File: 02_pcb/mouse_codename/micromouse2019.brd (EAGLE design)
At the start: 45 x 50 mm, 75 parts

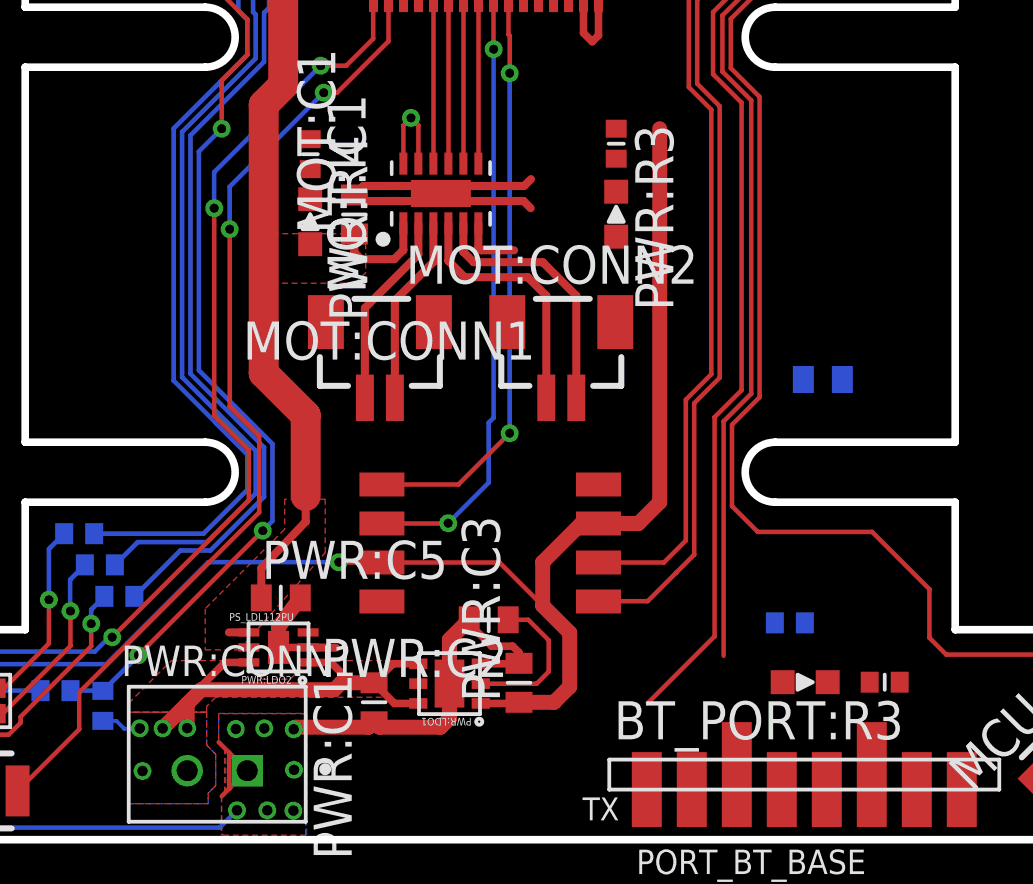
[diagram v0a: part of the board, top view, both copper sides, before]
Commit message: lib updated
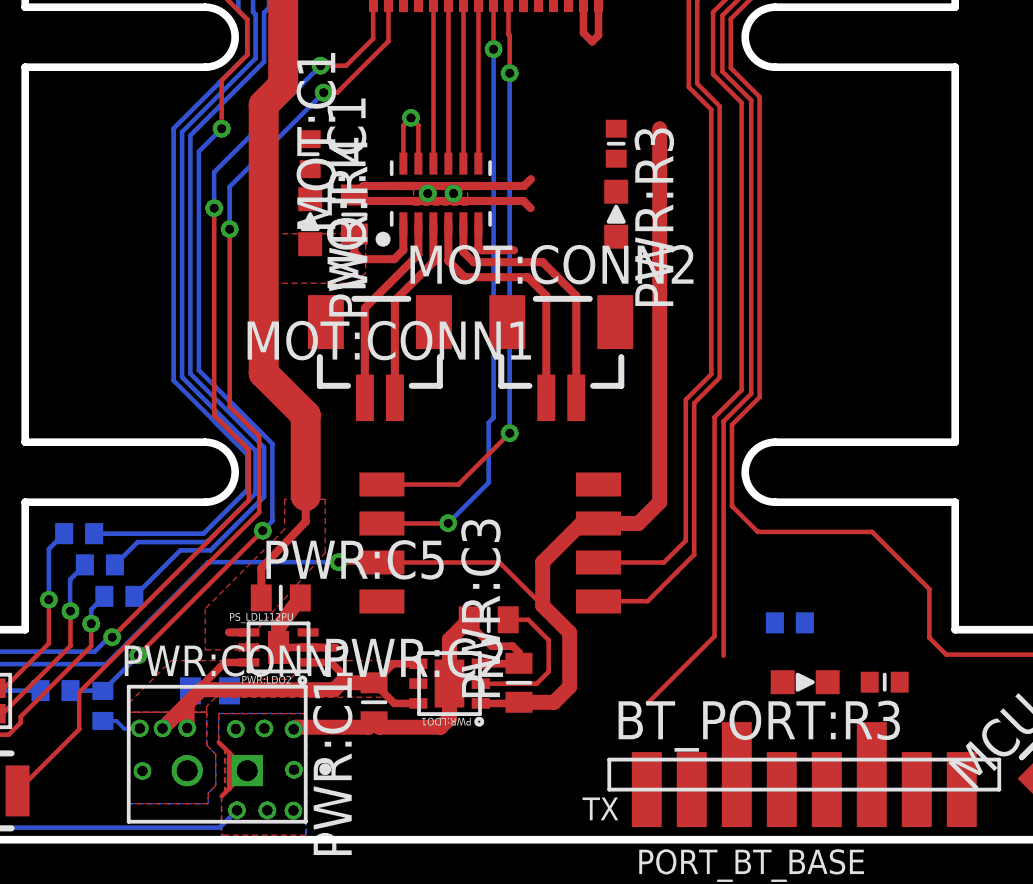
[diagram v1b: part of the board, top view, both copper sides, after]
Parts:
- moved PWR:C4 22.9 mm to (13.2, 4.96), turned to 180 degrees
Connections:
- net GND: no longer MOT:IC1.13
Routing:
- net GND: track 58.2 -> 67.9 mm, vias 8 -> 10
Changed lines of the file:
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@@
 <drawing>
 <settings>
-<setting alwaysvectorfont="yes"/>
+<setting alwaysvectorfont="no"/>
 <setting verticaltext="up"/>
 </settings>
@@
 <attribute name="VALUE" x="25.365" y="4.595" size="1.27" layer="27" rot="R90"/>
 </element>
-<element name="PWR:C4" library="0-micromouse2019" package="C0402" package3d_urn="urn:adsk.eagle:package:23626/2" value="1u" x="33.59" y="15.34" smashed="yes" rot="MR0">
-<attribute name="NAME" x="34.225" y="15.975" size="1.27" layer="26" rot="MR0"/>
-<attribute name="SPICEPREFIX" value="C" x="33.59" y="15.34" size="1.778" layer="28" rot="MR0" display="off"/>
-<attribute name="VALUE" x="34.225" y="13.435" size="1.27" layer="28" rot="MR0"/>
+<element name="PWR:C4" library="0-micromouse2019" package="C0402" package3d_urn="urn:adsk.eagle:package:23626/2" value="1u" x="13.16" y="4.96" smashed="yes" rot="MR180">
+<attribute name="NAME" x="12.525" y="4.325" size="1.27" layer="26" rot="MR180"/>
+<attribute name="SPICEPREFIX" value="C" x="13.16" y="4.96" size="1.778" layer="28" rot="MR180" display="off"/>
+<attribute name="VALUE" x="12.525" y="6.865" size="1.27" layer="28" rot="MR180"/>
 </element>
 <element name="PWR:C5" library="0-micromouse2019" package="C0402" package3d_urn="urn:adsk.eagle:package:23626/2" value="10u" x="15.52" y="8.06" smashed="yes">
@@
 <contactref element="MCU:J1" pad="3"/>
 <contactref element="MOT:C1" pad="2"/>
-<contactref element="MOT:IC1" pad="13"/>
 <contactref element="MOT:IC1" pad="14"/>
 <contactref element="MOT:IC1" pad="16"/>
@@
 <wire x1="15.45" y1="7.1" x2="16.17" y2="8.06" width="0.5" layer="1"/>
 <wire x1="16.4315" y1="6.409" x2="17.35" y2="6.4" width="0.27" layer="1"/>
-<polygon width="0.1524" layer="16" pour="cutout" rank="3">
+<polygon width="0.1524" layer="16" pour="cutout" isolate="0.3048" rank="3">
 <vertex x="0" y="0"/>
 <vertex x="45" y="0"/>
@@
 <contactref element="MCU:R8" pad="2"/>
 <contactref element="MCU:R9" pad="2"/>
+<via x="20.42" y="21.54" extent="1-16" drill="0.3" diameter="0.6"/>
+<via x="21.28" y="21.54" extent="1-16" drill="0.3" diameter="0.6"/>
+<polygon width="0.1" layer="1" spacing="0.5" isolate="0.254">
+<vertex x="19.95" y="21.9"/>
+<vertex x="21.75" y="21.9"/>
+<vertex x="21.75" y="21.15"/>
+<vertex x="19.95" y="21.15"/>
+</polygon>
+<wire x1="19.4874" y1="21.29" x2="22.2246" y2="21.29" width="0.27" layer="1"/>
+<wire x1="19.4874" y1="21.79" x2="22.2246" y2="21.79" width="0.27" layer="1"/>
+<wire x1="22.2246" y1="21.29" x2="21.53" y2="21.29" width="0.27" layer="1"/>
+<wire x1="21.53" y1="21.29" x2="21.285" y2="21.535" width="0.27" layer="1"/>
+<wire x1="21.285" y1="21.535" x2="21.28" y2="21.54" width="0.27" layer="1"/>
+<wire x1="22.2246" y1="21.79" x2="21.54" y2="21.79" width="0.27" layer="1"/>
+<wire x1="21.54" y1="21.79" x2="21.285" y2="21.535" width="0.27" layer="1"/>
+<wire x1="20.42" y1="21.54" x2="20.17" y2="21.29" width="0.27" layer="1"/>
+<wire x1="20.17" y1="21.29" x2="19.4874" y2="21.29" width="0.27" layer="1"/>
+<wire x1="20.42" y1="21.54" x2="20.17" y2="21.79" width="0.27" layer="1"/>
+<wire x1="20.17" y1="21.79" x2="19.4874" y2="21.79" width="0.27" layer="1"/>
 <wire x1="38" y1="36.7" x2="38" y2="38.3" width="0" layer="19" extent="16-16"/>
 <wire x1="38" y1="40" x2="38" y2="38.3" width="0" layer="19" extent="16-16"/>
@@
 <wire x1="9.8" y1="47.7" x2="9.75" y2="46.2" width="0" layer="19" extent="16-16"/>
 <wire x1="16.5" y1="23.35" x2="18.54" y2="28.74" width="0" layer="19" extent="1-16"/>
-<wire x1="18.273" y1="21.79" x2="16.5" y2="23.35" width="0" layer="19" extent="1-1"/>
-<wire x1="20.856" y1="21.54" x2="19.4874" y2="21.79" width="0" layer="19" extent="1-1"/>
-<wire x1="22.2246" y1="21.79" x2="20.856" y2="21.54" width="0" layer="19" extent="1-1"/>
-<wire x1="23.61" y1="21.29" x2="23.63" y2="21.79" width="0" layer="19" extent="1-1"/>
+<wire x1="17.973" y1="21.49" x2="16.5" y2="23.35" width="0" layer="19" extent="1-1"/>
 <wire x1="22.106" y1="20.5444" x2="22.2246" y2="21.29" width="0" layer="19" extent="1-1"/>
 <wire x1="26.7" y1="23.7" x2="23.86" y2="22.02" width="0" layer="19" extent="1-1"/>
 <wire x1="26.11" y1="11.84" x2="23.297" y2="19.647" width="0" layer="19" extent="1-1"/>
 <wire x1="23.25" y1="6.45" x2="26.11" y2="11.84" width="0" layer="19" extent="1-1"/>
-<wire x1="18.89" y1="7.94" x2="21.144" y2="6.674" width="0" layer="19" extent="1-1"/>
-<wire x1="17.35" y1="6.4" x2="18.89" y2="7.94" width="0" layer="19" extent="1-1"/>
-<wire x1="32.94" y1="15.34" x2="26.11" y2="11.84" width="0" layer="19" extent="1-16"/>
+<wire x1="13.81" y1="4.96" x2="14.02" y2="3.69" width="0" layer="19" extent="16-16"/>
+<wire x1="15.444" y1="6.409" x2="13.81" y2="4.96" width="0" layer="19" extent="1-16"/>
+<wire x1="18.89" y1="7.94" x2="17.35" y2="6.4" width="0" layer="19" extent="1-1"/>
 <wire x1="15.75" y1="56.8" x2="20.385" y2="48.379" width="0" layer="19" extent="1-16"/>
 <wire x1="14.7" y1="56.8" x2="15.75" y2="56.8" width="0" layer="19" extent="16-16"/>
 <wire x1="13.6" y1="56.8" x2="14.7" y2="56.8" width="0" layer="19" extent="16-16"/>
-<wire x1="36.15" y1="5.25" x2="32.94" y2="15.34" width="0" layer="19" extent="1-16"/>
+<wire x1="36.15" y1="5.25" x2="26.11" y2="11.84" width="0" layer="19" extent="1-1"/>
 <wire x1="36.72" y1="1.67" x2="36.15" y2="5.25" width="0" layer="19" extent="1-1"/>
 </signal>
@@
 <contactref element="PWR:LDO1" pad="4"/>
 <contactref element="PWR:LDO1" pad="6"/>
-<wire x1="20.1026" y1="5.8634" x2="34.24" y2="15.34" width="0" layer="19" extent="1-16"/>
+<wire x1="12.87" y1="5" x2="12.51" y2="4.96" width="0" layer="19" extent="1-16"/>
 </signal>
 <signal name="DRV_A_IN1">
